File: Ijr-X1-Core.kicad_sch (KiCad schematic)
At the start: 19 parts, among them J1 USB-C_PWR_IN, J2 USB-C_CPU_PROG, J3 USB-C_UART_BRIDGE, U1 RP2040, U2 W25Q16JVSSIQ

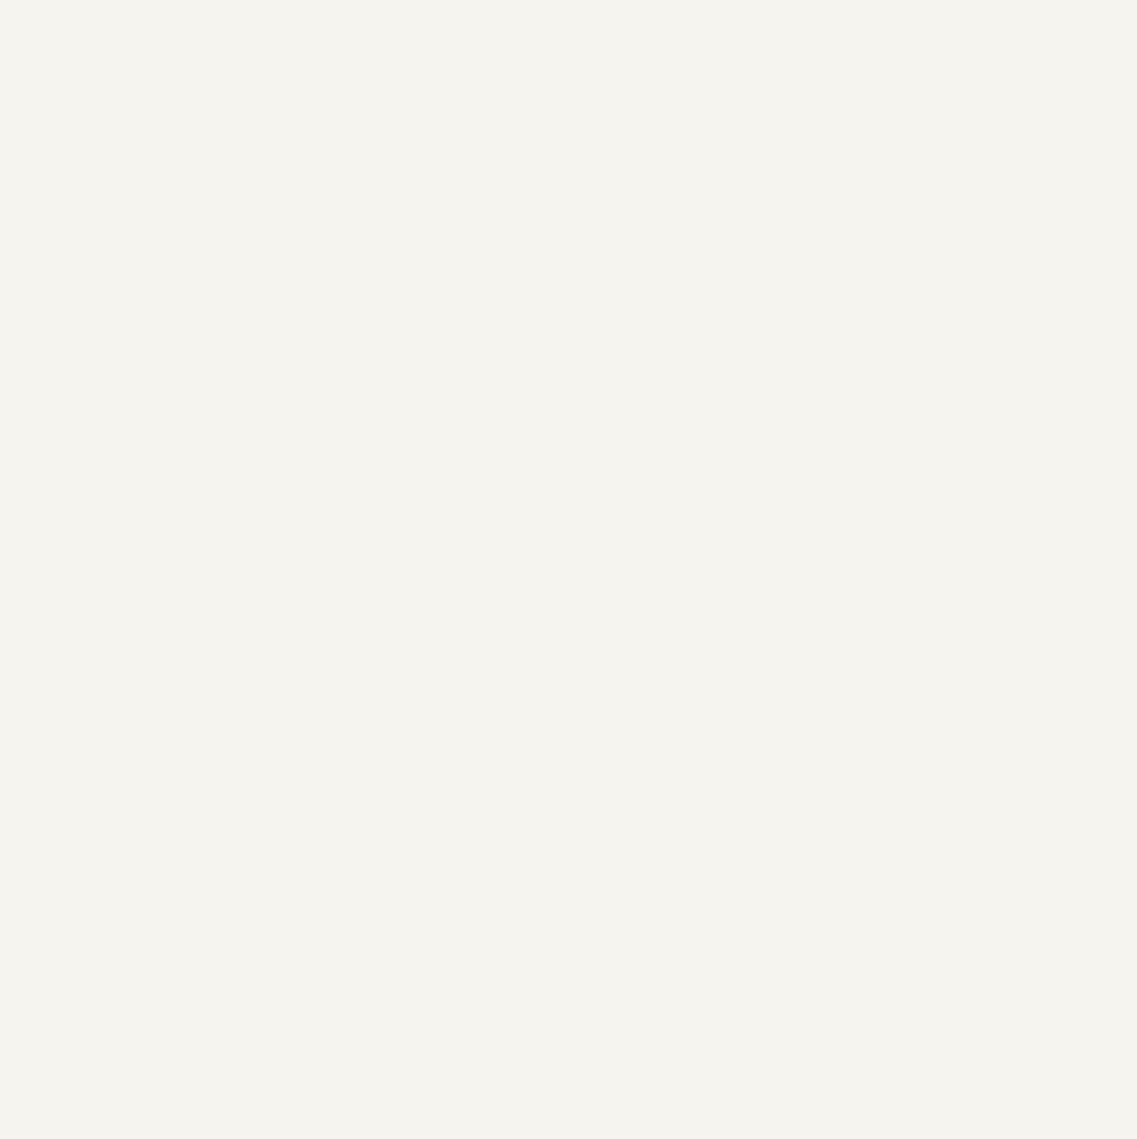
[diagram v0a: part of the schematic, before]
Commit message: Some updates1
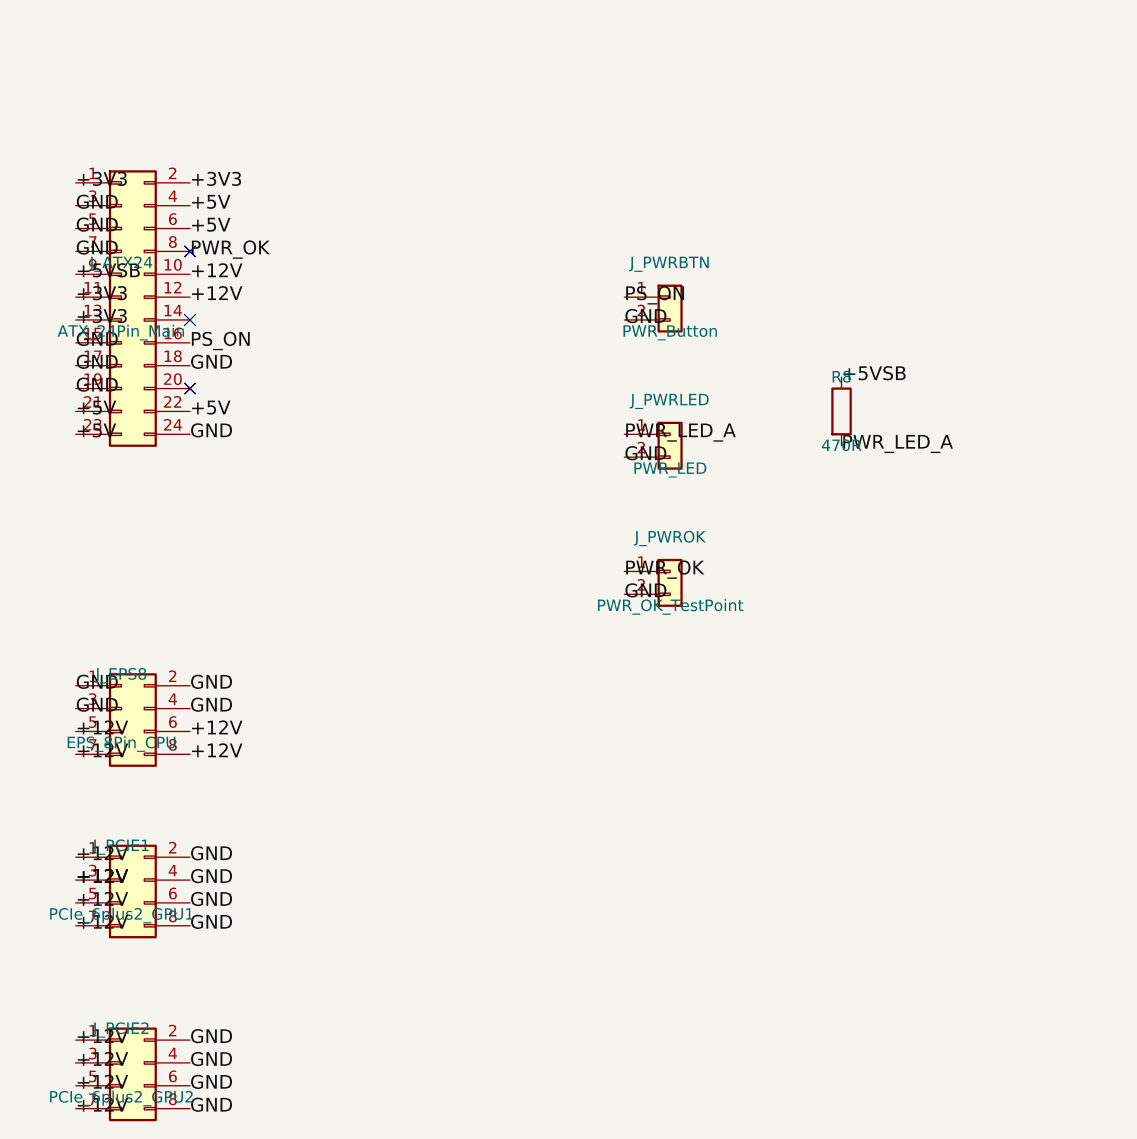
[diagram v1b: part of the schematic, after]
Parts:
- added J_ATX24: ATX_24Pin_Main, symbol Connector_Generic:Conn_02x12_Odd_Even
- added J_EPS8: EPS_8Pin_CPU, symbol Connector_Generic:Conn_02x04_Odd_Even
- added J_PCIE1: PCIe_6plus2_GPU1, symbol Connector_Generic:Conn_02x04_Odd_Even
- added J_PCIE2: PCIe_6plus2_GPU2, symbol Connector_Generic:Conn_02x04_Odd_Even
- added J_PWRBTN: PWR_Button, symbol Connector_Generic:Conn_01x02
- added J_PWRLED: PWR_LED, symbol Connector_Generic:Conn_01x02
- added J_PWROK: PWR_OK_TestPoint, symbol Connector_Generic:Conn_01x02
- added R8: 470R, symbol Device:R
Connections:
- net +3V3: now also J_ATX24.1 (Pin_1), J_ATX24.11 (Pin_11), J_ATX24.13 (Pin_13), J_ATX24.2 (Pin_2)
- net +5V: now also J_ATX24.21 (Pin_21), J_ATX24.22 (Pin_22), J_ATX24.23 (Pin_23), J_ATX24.4 (Pin_4), J_ATX24.6 (Pin_6)
- net GND: now also J_ATX24.15 (Pin_15), J_ATX24.17 (Pin_17), J_ATX24.18 (Pin_18), J_ATX24.19 (Pin_19), J_ATX24.24 (Pin_24), J_ATX24.3 (Pin_3), J_ATX24.5 (Pin_5), J_ATX24.7 (Pin_7), J_EPS8.1 (Pin_1), J_EPS8.2 (Pin_2), J_EPS8.3 (Pin_3), J_EPS8.4 (Pin_4), J_PCIE1.2 (Pin_2), J_PCIE1.4 (Pin_4), J_PCIE1.6 (Pin_6), J_PCIE1.8 (Pin_8), J_PCIE2.2 (Pin_2), J_PCIE2.4 (Pin_4), J_PCIE2.6 (Pin_6), J_PCIE2.8 (Pin_8), J_PWRBTN.2 (Pin_2), J_PWRLED.2 (Pin_2), J_PWROK.2 (Pin_2)
- new net +12V: J_ATX24.10 (Pin_10), J_ATX24.12 (Pin_12), J_EPS8.5 (Pin_5), J_EPS8.6 (Pin_6), J_EPS8.7 (Pin_7), J_EPS8.8 (Pin_8), J_PCIE1.1 (Pin_1), J_PCIE1.3 (Pin_3), J_PCIE1.5 (Pin_5), J_PCIE1.7 (Pin_7), J_PCIE2.1 (Pin_1), J_PCIE2.3 (Pin_3), J_PCIE2.5 (Pin_5), J_PCIE2.7 (Pin_7)
- new net +5VSB: J_ATX24.9 (Pin_9), R8.1
- new net PS_ON: J_ATX24.16 (Pin_16), J_PWRBTN.1 (Pin_1)
- new net PWR_LED_A: J_PWRLED.1 (Pin_1), R8.2
- new net PWR_OK: J_ATX24.8 (Pin_8), J_PWROK.1 (Pin_1)
- no-connect marks 26 -> 29

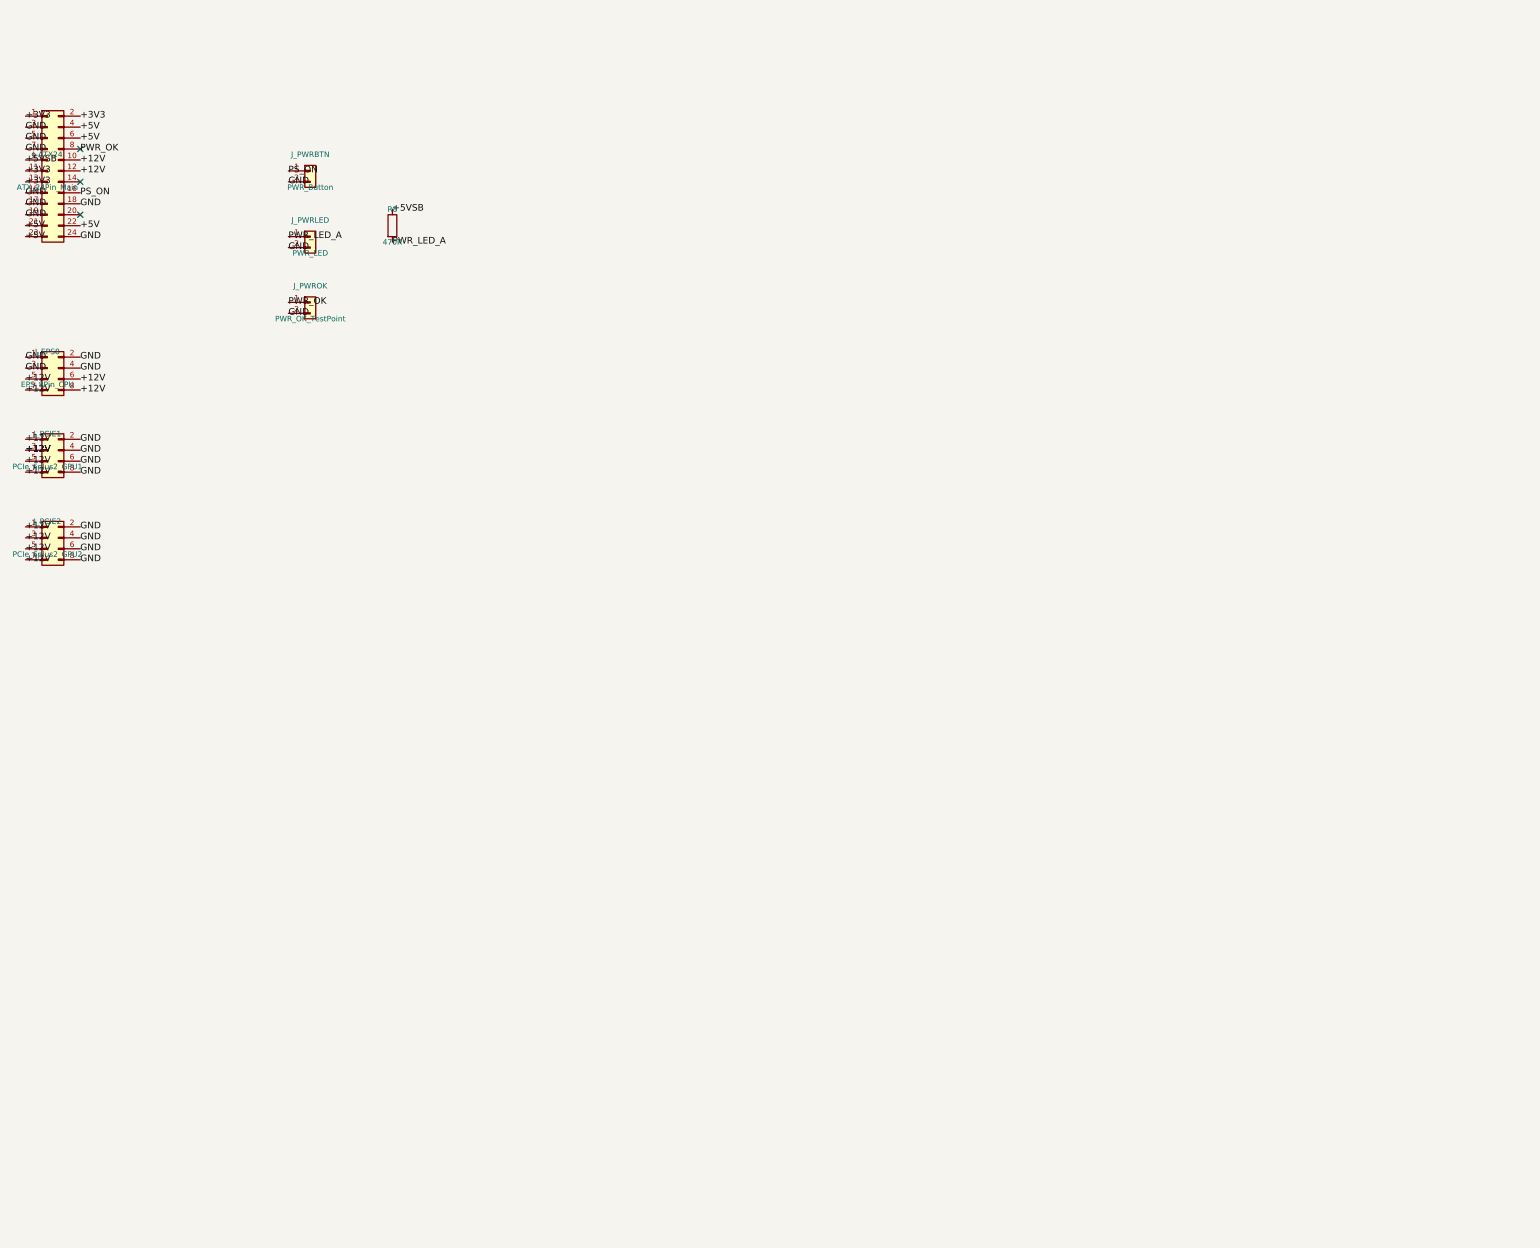
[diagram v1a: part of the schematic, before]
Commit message: Some updates1
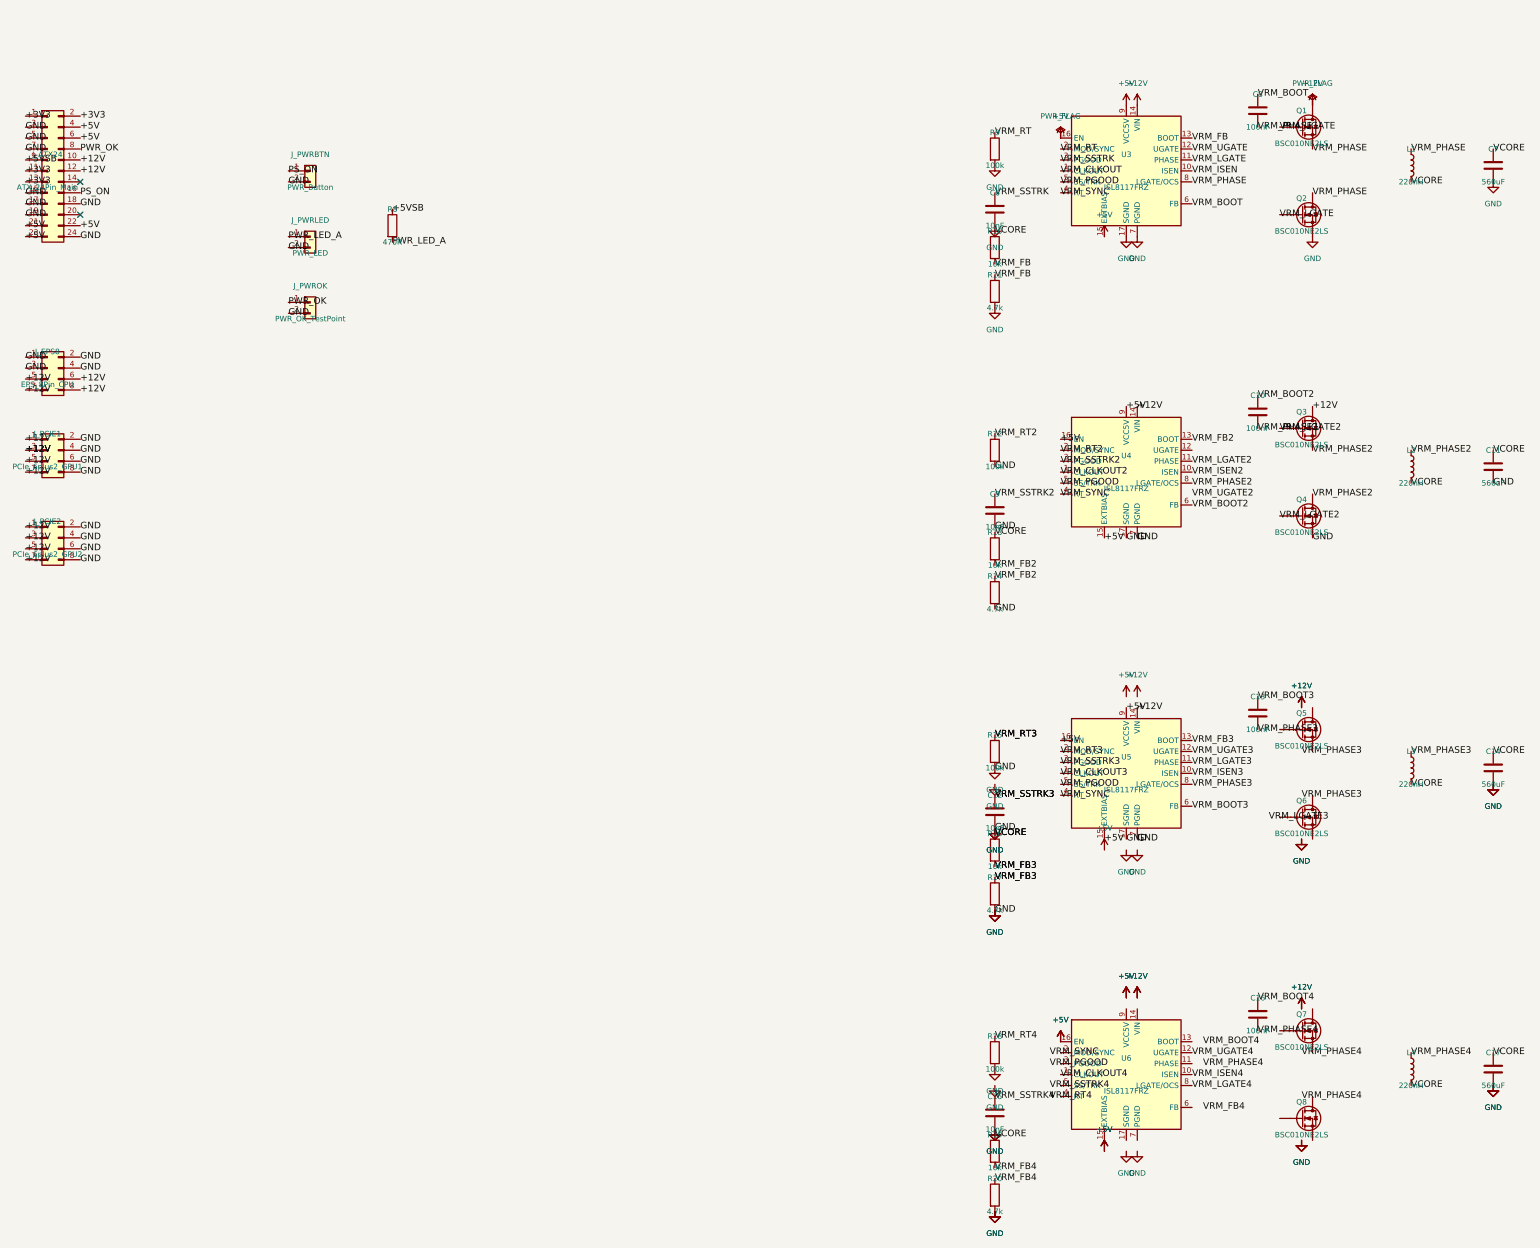
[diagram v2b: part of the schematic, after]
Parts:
- added C10, C13, C16, C8: 100nF, symbol Device:C
- added C11, C14, C17, C7: 560uF, symbol Device:C
- added C12, C15, C6, C9: 10nF, symbol Device:C
- added L1, L2, L3, L4: 220nH, symbol Device:L
- added Q1, Q2, Q3, Q4, Q5, Q6, Q7, Q8: BSC010NE2LS, symbol Device:Q_NMOS
- added R10, R13, R16, R19: 10k, symbol Device:R
- added R11, R14, R17, R20: 4.7k, symbol Device:R
- added R12, R15, R18, R9: 100k, symbol Device:R
- added U3, U4, U5, U6: ISL8117FRZ, symbol Regulator_Switching:ISL8117FRZ
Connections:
- net +12V: now also Q1.D, Q3.D, U3.14 (VIN), U4.14 (VIN), U5.14 (VIN)
- net +5V: now also U3.15 (EXTBIAS), U3.16 (EN), U3.9 (VCC5V), U4.15 (EXTBIAS), U4.16 (EN), U4.9 (VCC5V), U5.15 (EXTBIAS), U5.16 (EN), U5.9 (VCC5V), U6.16 (EN)
- net GND: now also C11.2, C12.2, C14.2, C15.2, C17.2, C6.2, C7.2, C9.2, Q2.S, Q4.S, R11.2, R12.2, R14.2, R15.2, R17.2, R18.2, R20.2, R9.2, U3.17 (SGND), U3.7 (PGND), U4.17 (SGND), U4.7 (PGND), U5.17 (SGND), U5.7 (PGND)
- new net VCORE: C11.1, C14.1, C17.1, C7.1, L1.2, L2.2, L3.2, L4.2, R10.1, R13.1, R16.1, R19.1
- new net VRM_BOOT: C8.1, U3.6 (FB)
- new net VRM_BOOT2: C10.1, U4.6 (FB)
- new net VRM_BOOT3: C13.1, U5.6 (FB)
- new net VRM_BOOT4: C16.1
- new net VRM_CLKOUT: U3.1 (CLKOUT)
- new net VRM_CLKOUT2: U4.1 (CLKOUT)
- new net VRM_CLKOUT3: U5.1 (CLKOUT)
- new net VRM_CLKOUT4: U6.1 (CLKOUT)
- new net VRM_FB: R10.2, R11.1, U3.13 (BOOT)
- new net VRM_FB2: R13.2, R14.1, U4.13 (BOOT)
- new net VRM_FB3: R16.2, R17.1, U5.13 (BOOT)
- new net VRM_FB4: R19.2, R20.1
- new net VRM_ISEN: U3.10 (ISEN)
- new net VRM_ISEN2: U4.10 (ISEN)
- new net VRM_ISEN3: U5.10 (ISEN)
- new net VRM_ISEN4: U6.10 (ISEN)
- new net VRM_LGATE: Q2.G, U3.11 (PHASE)
- new net VRM_LGATE2: Q4.G, U4.11 (PHASE)
- new net VRM_LGATE3: U5.11 (PHASE)
- new net VRM_LGATE4: U6.8 (LGATE/OCS)
- new net VRM_PGOOD: U3.5 (SS/TRK), U4.5 (SS/TRK), U5.5 (SS/TRK)
- new net VRM_PHASE: C8.2, L1.1, Q1.S, Q2.D, U3.8 (LGATE/OCS)
- new net VRM_PHASE2: C10.2, L2.1, Q3.S, Q4.D, U4.8 (LGATE/OCS)
- new net VRM_PHASE3: C13.2, L3.1, U5.8 (LGATE/OCS)
- new net VRM_PHASE4: C16.2, L4.1
- new net VRM_RT: R9.1, U3.2 (MOD/SYNC)
- new net VRM_RT2: R12.1, U4.2 (MOD/SYNC)
- new net VRM_RT3: R15.1, U5.2 (MOD/SYNC)
- new net VRM_RT4: R18.1
- new net VRM_SSTRK: C6.1, U3.3 (PGOOD)
- new net VRM_SSTRK2: C9.1, U4.3 (PGOOD)
- new net VRM_SSTRK3: C12.1, U5.3 (PGOOD)
- new net VRM_SSTRK4: C15.1
- new net VRM_SYNC: U3.4 (RT), U4.4 (RT), U5.4 (RT)
- new net VRM_UGATE: Q1.G, U3.12 (UGATE)
- new net VRM_UGATE2: Q3.G
- new net VRM_UGATE3: U5.12 (UGATE)
- new net VRM_UGATE4: U6.12 (UGATE)
- no-connect marks 29 -> 28
